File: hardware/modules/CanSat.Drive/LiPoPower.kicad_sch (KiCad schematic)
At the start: 26 parts, among them SW901 Power Switch, U901 INA226, U902 TPS63070RNMR, U903 INA226

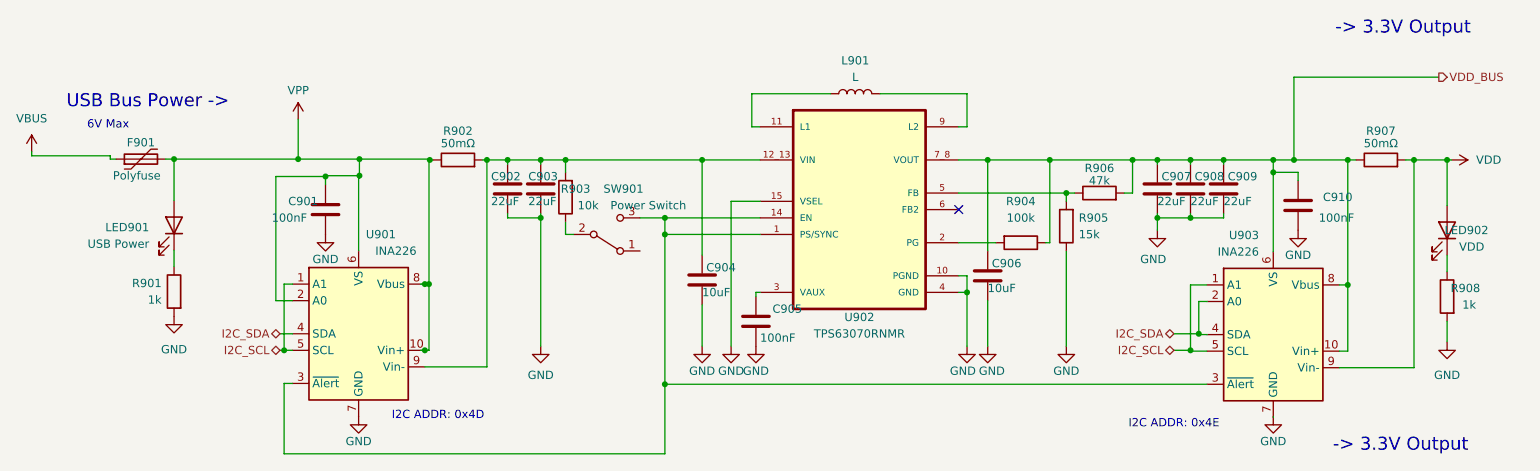
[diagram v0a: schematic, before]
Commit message: 一旦
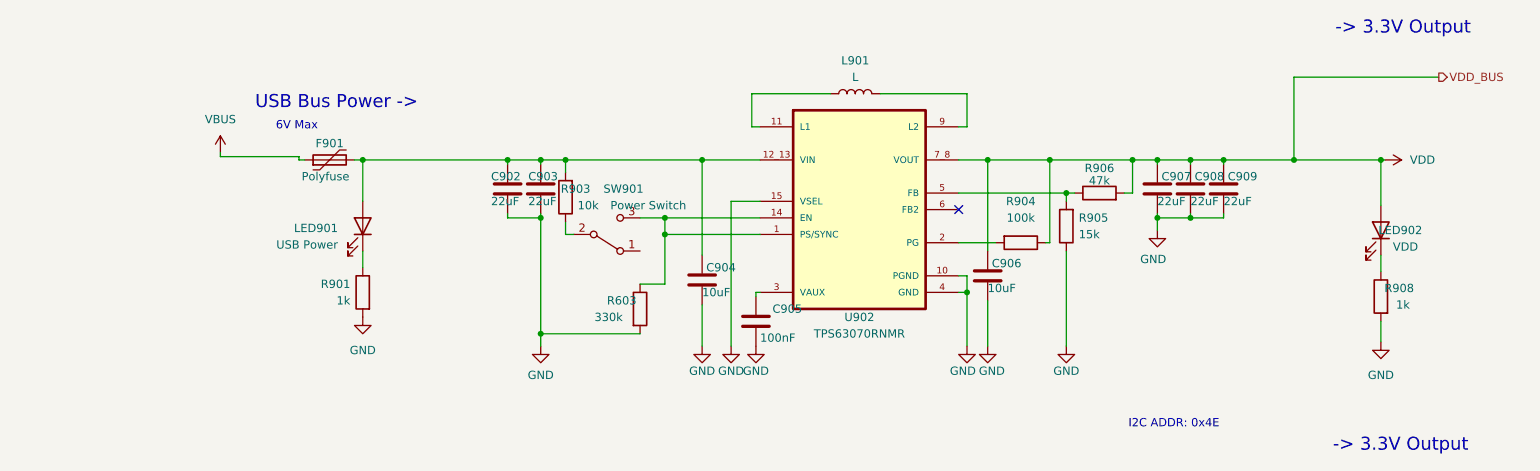
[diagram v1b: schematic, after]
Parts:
- removed C901, C910: 100nF, Capacitor_SMD:C_0402_1005Metric, symbol Device:C
- removed R902, R907: 50mΩ, Resistor_SMD:R_0805_2012Metric, symbol Device:R
- removed U901, U903: INA226, Package_SO:VSSOP-10_3x3mm_P0.5mm, symbol Sensor_Energy:INA226
- added R603: 330k, Resistor_SMD:R_0402_1005Metric, symbol Device:R
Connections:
- net VDD_BUS is gone; now on net VDD: C906.1, C907.1, C908.1, C909.1, R904.1, R906.2, U902.7_8 (VOUT)
- net VPP is gone; now on an unnamed net: F901.2, LED901.2 (A)
- net GND: now also R603.2
- net at SW901.3 (C), U902.1 (PS/SYNC), U902.14 (EN): now also R603.1
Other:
- note removed: "I2C ADDR: 0x4D"
- moved on the sheet: F901, LED901, LED902, R901, R908

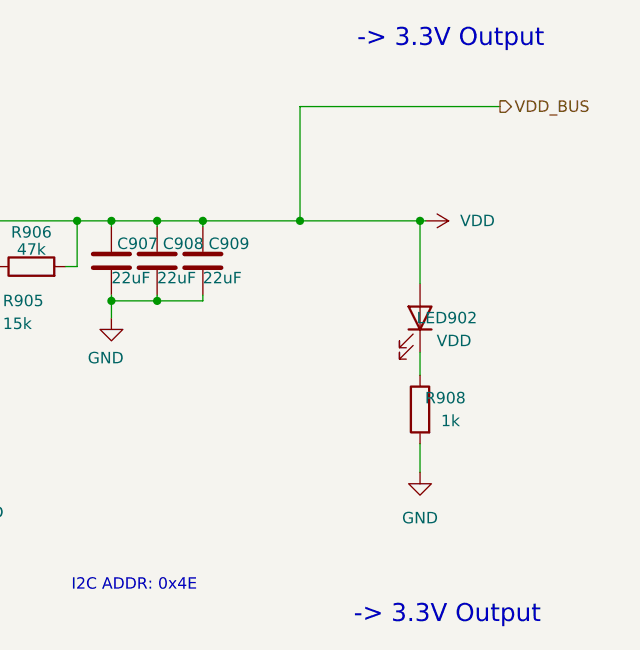
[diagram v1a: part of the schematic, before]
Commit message: デザインルールチェックまで完了
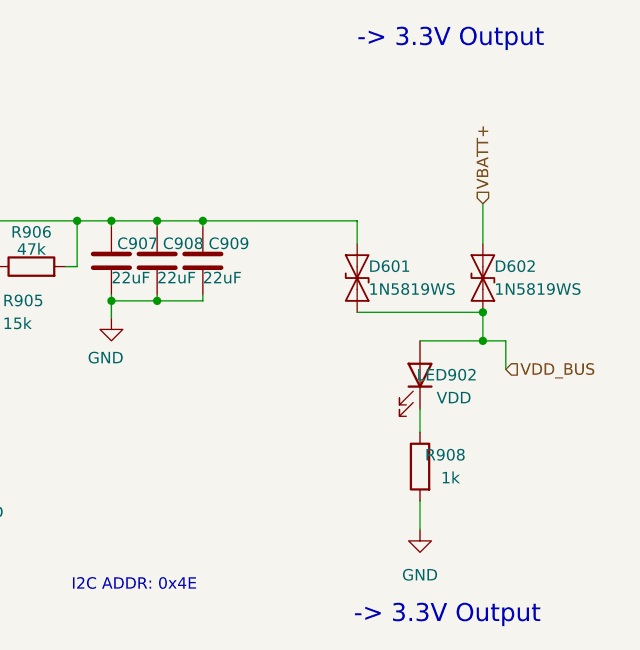
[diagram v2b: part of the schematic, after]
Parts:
- added D601, D602: 1N5819WS, Diode_SMD:D_SOD-323, symbol Diode:ESD9B5.0ST5G
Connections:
- net VDD: no longer names the net of C906.1, C907.1, C908.1, C909.1, R904.1, R906.2, U902.7_8 (VOUT)
- net VDD: now also D601.2 (A2); no longer LED902.2 (A)
- new net VBATT+: D602.2 (A2)
- new net VDD_BUS: D601.1 (A1), D602.1 (A1), LED902.2 (A)
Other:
- moved on the sheet: LED902, R908

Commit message: コネクタのの位置修正，LCSC番号間違い修正
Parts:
- R603: LCSC C23137 -> C25778
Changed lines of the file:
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@@
 			)
 		)
-		(property "LCSC" "C23137"
+		(property "LCSC" "C25778"
 			(at 127 106.68 0)
 			(effects

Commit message: 最終確認
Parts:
- F901: LCSC C883133 -> C883133
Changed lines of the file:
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@@
 			)
 		)
-		(property "LCSC" " C883133"
+		(property "LCSC" "C883133"
 			(at 79.375 83.82 0)
 			(effects
